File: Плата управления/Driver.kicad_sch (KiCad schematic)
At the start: 30 parts, among them U1 IR2184, U2 IR2184, U3 IR2184

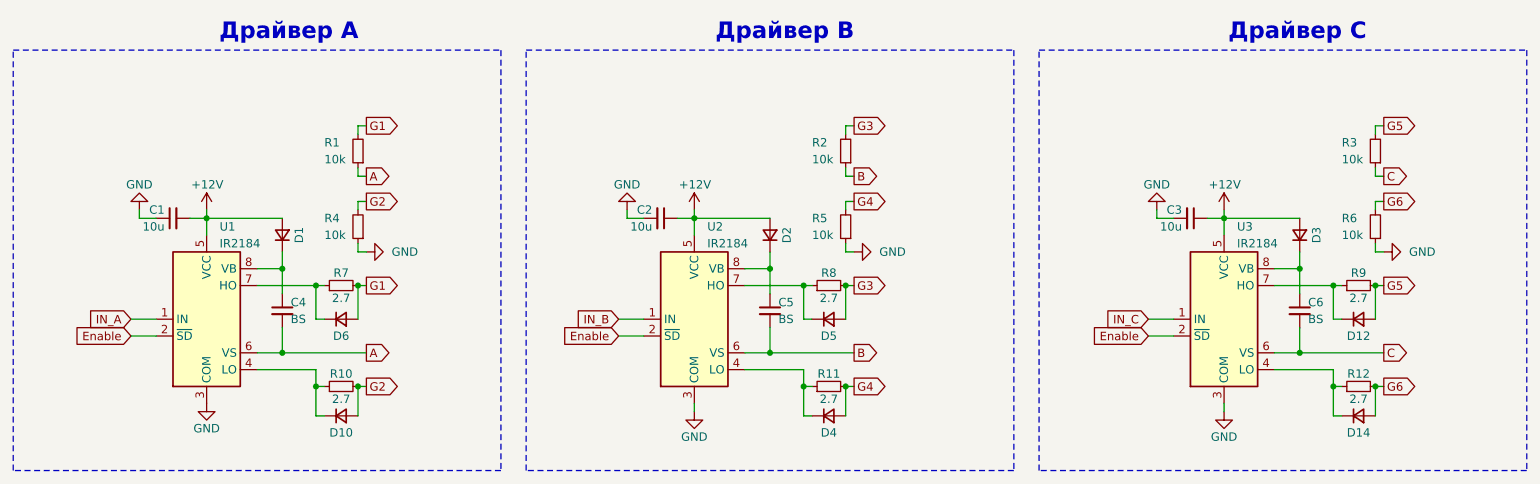
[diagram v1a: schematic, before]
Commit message: Новые драйвера и разъёмы
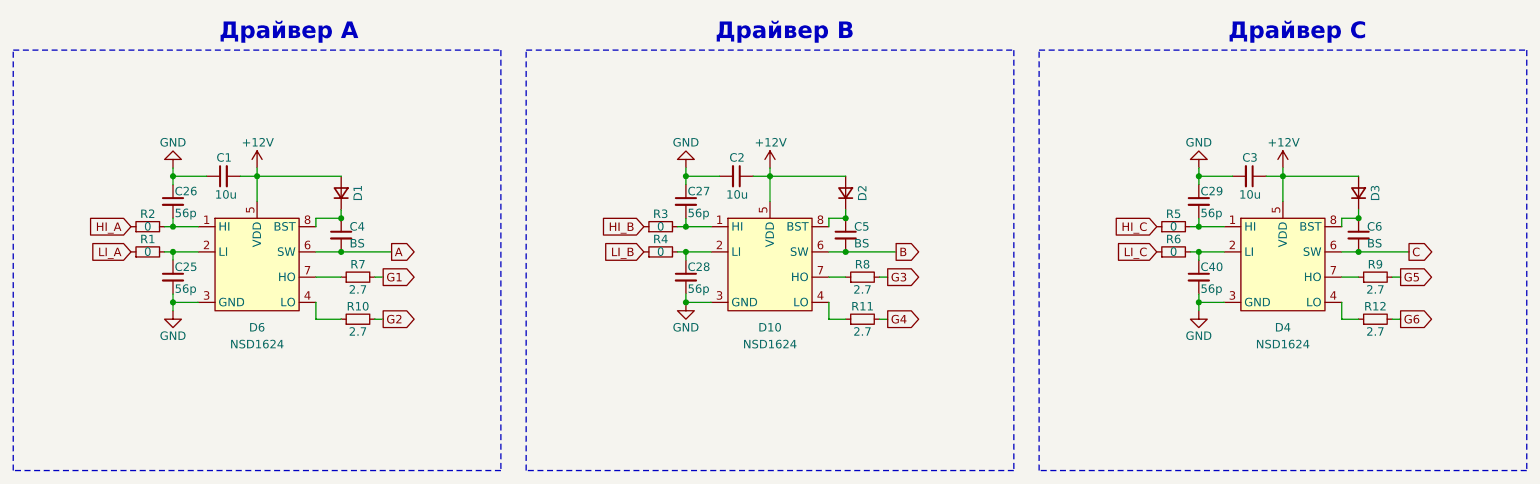
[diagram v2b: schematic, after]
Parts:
- removed D10, D12, D14, D4, D5, D6: D_Small, Diode_SMD:D_SMA_Handsoldering, symbol Device:D_Small
- removed U1, U2, U3: IR2184, Package_SO:SO-8_3.9x4.9mm_P1.27mm, symbol Driver_FET:IR2184
- added C25, C26, C27, C28, C29, C40: 56p, Capacitor_SMD:C_0603_1608Metric_Pad1.08x0.95mm_HandSolder, symbol Device:C_Small
- added D10, D4, D6: NSD1624, Package_SO:SOIC-8_3.9x4.9mm_P1.27mm, symbol Novosense:NSD1624
- R1, R2, R3, R4, R5, R6: value 10k -> 0
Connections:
- net +12V: now also D10.5 (VDD), D4.5 (VDD), D6.5 (VDD)
- net A: now also D6.6 (SW); no longer R1.1
- net B: now also D10.6 (SW); no longer R2.1
- net C: now also D4.6 (SW); no longer R3.1
- net G1: no longer R1.2
- net G2: no longer R4.2
- net G3: no longer R2.2
- net G4: no longer R5.2
- net G5: no longer R3.2
- net G6: no longer R6.2
- net GND: now also C25.2, C26.1, C27.1, C28.2, C29.1, C40.2, D10.3 (GND), D4.3 (GND), D6.3 (GND); no longer R4.1, R5.1, R6.1
- net at R12.1: now also D4.4 (LO)
- net at R8.1: now also D10.7 (HO)
- net at R11.1: now also D10.4 (LO)
- net at C5.1, D2.1 (K): now also D10.8 (BST)
- net at C6.1, D3.1 (K): now also D4.8 (BST)
- net at R7.1: now also D6.7 (HO)
- net at R9.1: now also D4.7 (HO)
- net at R10.1: now also D6.4 (LO)
- net at C4.1, D1.1 (K): now also D6.8 (BST)
- new net: C26.2, D6.1 (HI), R2.2
- new net: C29.2, D4.1 (HI), R5.2
- new net: C40.1, D4.2 (LI), R6.2
- new net: C25.1, D6.2 (LI), R1.2
- new net: C28.1, D10.2 (LI), R4.2
- new net: C27.2, D10.1 (HI), R3.2
- new net HI_A: R2.1
- new net HI_B: R3.1
- new net HI_C: R5.1
- new net LI_A: R1.1
- new net LI_B: R4.1
- new net LI_C: R6.1
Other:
- moved on the sheet: C1, C2, C3, C4, C5, C6, D1, D2, D3, R10, R11, R12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
